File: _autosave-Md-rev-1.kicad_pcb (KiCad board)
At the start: 2 copper layers, 50 x 21.5 mm, 29 parts, among them J1 USB_C_Receptacle_USB2.0, J2 54-00177, U1 MCP73831-2-OT, U2 MAX9814

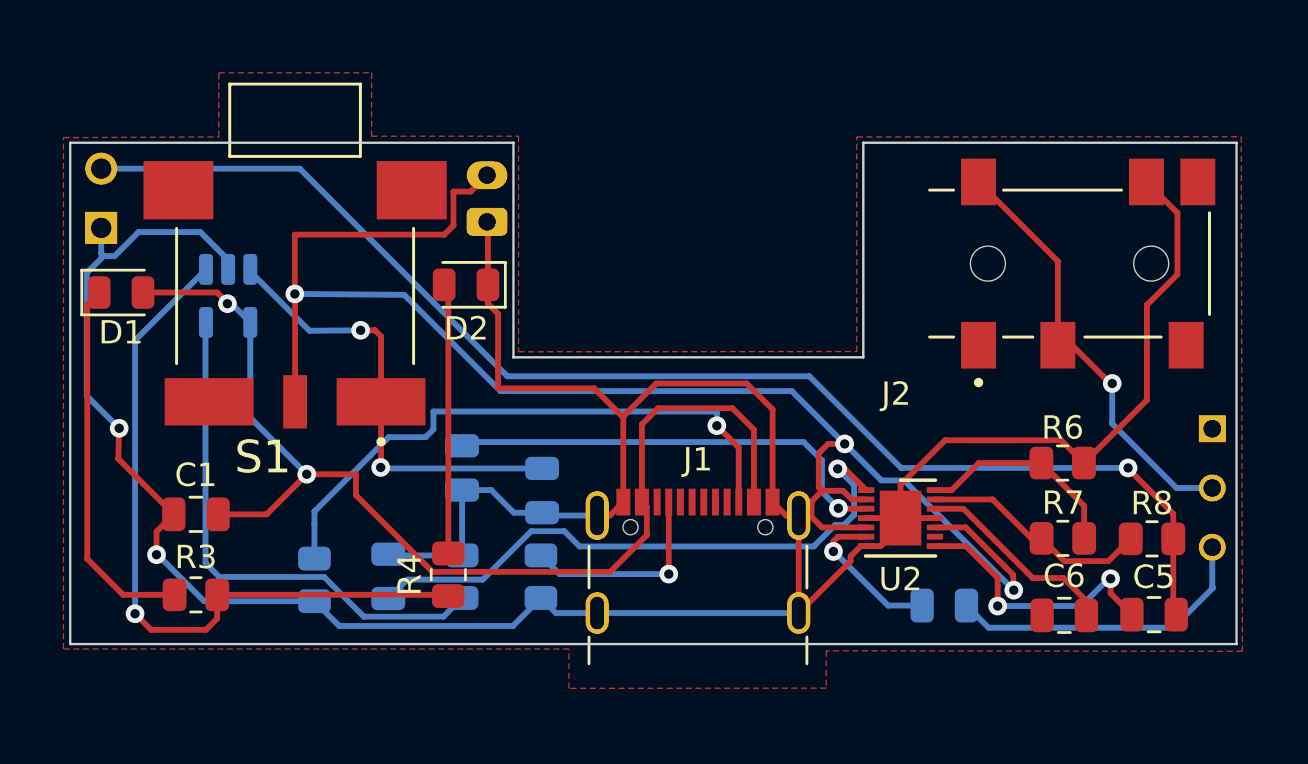
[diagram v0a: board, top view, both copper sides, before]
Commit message: updated the final PCB
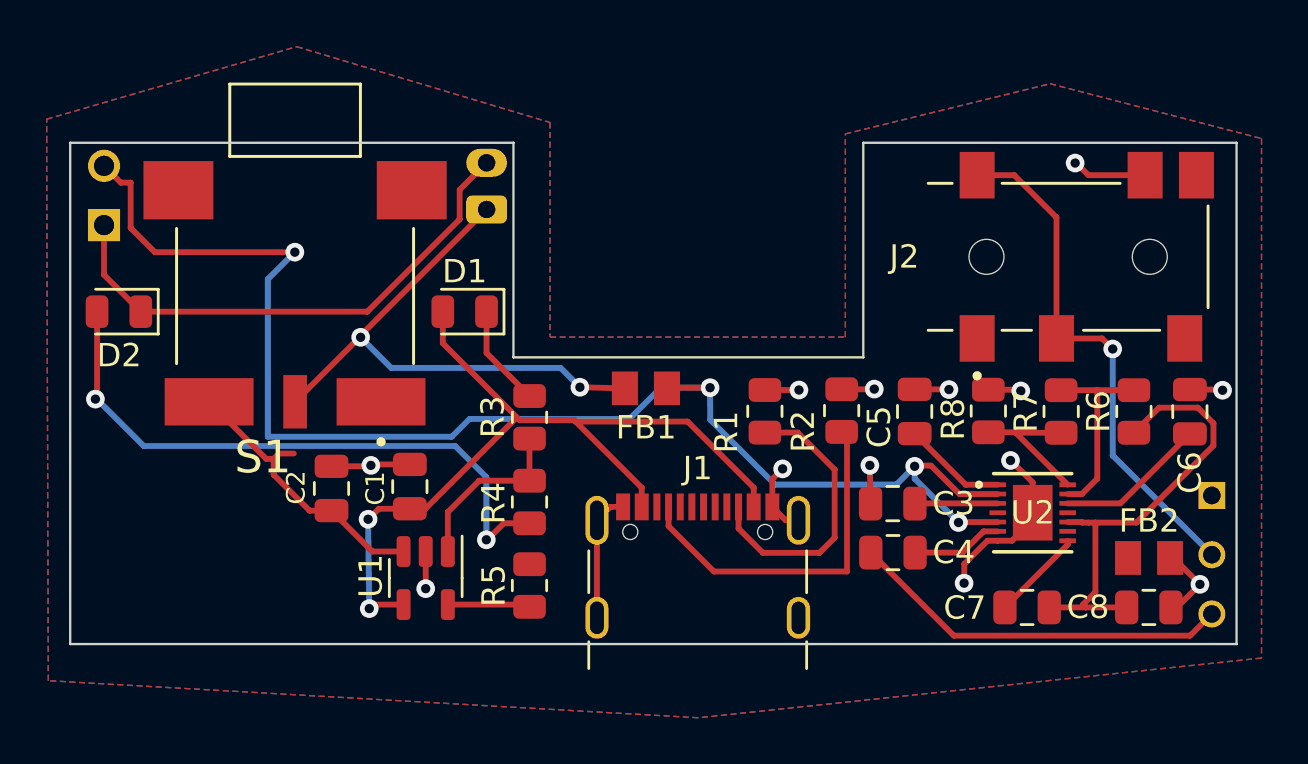
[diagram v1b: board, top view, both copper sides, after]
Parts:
- removed the ? at (179.0, 118.9)
- removed the ? at (147.9, 107.5)
- removed the ? at (179.0, 116.4)
- removed the ? at (131.3, 105.2)
- removed the ? at (179.0, 121.5)
- removed the ? at (147.9, 105.5)
- removed the ? at (131.3, 107.8)
- added ?: , , F.Cu at (178.9, 119.3)
- added ?: , , F.Cu at (178.9, 124.3)
- added ?: , , F.Cu at (131.4, 107.7)
- added ?: , , F.Cu at (147.8, 105.0)
- added ?: , , F.Cu at (131.4, 105.1)
- added ?: , , F.Cu at (147.8, 107.0)
- added ?: , , F.Cu at (178.9, 121.8)
- added C8: 2.2uF, Capacitor_SMD:C_0805_2012Metric, F.Cu at (176.2, 124.1)
- added FB1: FERRITE, LI0805H151R_10:IND_LI0805H151R-10_LRD, F.Cu at (154.7, 114.7)
- added FB2: FERRITE, LI0805H151R_10:IND_LI0805H151R-10_LRD, F.Cu at (176.2, 121.9)
- C2, R1, R2, R5, U1: moved to F.Cu
- C3: value 0.1uF -> 2.2uF; moved to F.Cu
- C4: value 2.2uF -> 10uF; moved to F.Cu
- C7: value 10uF -> 0.1uF; moved to F.Cu
- R6: value 100k -> 2.2K
- R8: value 2.2K -> 100k
- U2: value MAX9814 -> max9814etd+t; footprint Package_DFN_QFN:DFN-14-1EP_3x3mm_P0.4mm_EP1.78x2.35mm -> MAX9814etd+T:21-0137I_T1433-2_MXM
- moved C3 21.8 mm to (165.3, 119.6), turned to 0 degrees
- moved R1 20.6 mm to (159.8, 115.7), turned to 90 degrees
- moved C4 18.8 mm to (165.3, 121.7), turned to 0 degrees
- moved R3 16.2 mm to (149.7, 115.9), turned to 90 degrees
- moved D2 14.9 mm to (132.1, 111.4)
- moved U1 14.8 mm to (145.2, 122.8)
- moved D1 14.8 mm to (146.9, 111.4), turned to 180 degrees
- moved R2 14.7 mm to (163.1, 115.6), turned to 90 degrees
- moved C5 13.5 mm to (166.2, 115.7), turned to -90 degrees
- moved C6 10.3 mm to (178.0, 115.7), turned to -90 degrees
- moved C1 9.25 mm to (144.6, 118.9), turned to -90 degrees
- moved C2 9.03 mm to (141.2, 119.0), turned to 90 degrees
- moved R8 8.90 mm to (169.4, 115.6), turned to 90 degrees
- moved U2 5.67 mm to (171.3, 120.0)
- moved R7 5.44 mm to (172.5, 115.7), turned to -90 degrees
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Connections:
- C3 pad 2: Net-(U2-CT) -> Net-(U2-CG)
- C4 pad 1: GND -> /OUTPUT
- C4 pad 2: Net-(U2-CG) -> Net-(U2-MICOUT)
- C5 pad 1: Net-(C5-Pad1) -> GND
- C5 pad 2: Net-(U2-MICIN) -> Net-(U2-CT)
- C7 pad 1: Net-(U2-MICOUT) -> Net-(U2-MICIN)
- C7 pad 2: /OUTPUT -> VDD
- R6 pad 1: GND -> VDD
- R6 pad 2: Net-(U2-TH) -> Net-(U2-MICBIAS)
- R7 pad 1: Net-(U2-TH) -> Net-(U2-MICBIAS)
- R7 pad 2: Net-(U2-MICBIAS) -> Net-(U2-TH)
- R8 pad 1: Net-(C5-Pad1) -> Net-(U2-TH)
- R8 pad 2: Net-(U2-MICBIAS) -> GND
- S1 pad 1: Net-(U1-V_{BAT}) -> unconnected-(S1-Pad1)
- S1 pad 2: /GAIN -> /VBAT
- S1 pad 3: unconnected-(S1-Pad3) -> Net-(U1-V_{BAT})
- U2 pad 10: /GAIN -> VDD
- U2 pad 11: GND -> unconnected-(U2-NC-Pad11)
- U2 pad 2: /GAIN -> VDD
- U2 pad 4: GND -> unconnected-(U2-NC-Pad4)
- U2 pad 5: /GAIN -> VDD
- U2 pad 9: /A/R -> unconnected-(U2-A/R-Pad9)
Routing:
- net VDD: track 0.00 -> 81.8 mm, vias 0 -> 4
- net GND: track 134.2 -> 60.7 mm, vias 2 -> 13
- net /GAIN: track 67.5 -> 0.00 mm, vias 3 -> 0
- net Net-(C5-Pad1): track 57.0 -> 0.00 mm, vias 1 -> 0
- net /VBAT: track 0.00 -> 24.1 mm, vias 0 -> 2
- net Net-(U1-STAT): track 31.0 -> 7.55 mm, vias 1 -> 0
- net Net-(U2-CT): track 25.9 -> 4.47 mm, vias 1 -> 0
- net Net-(U1-PROG): track 22.6 -> 3.54 mm
- net Net-(U2-CG): track 19.4 -> 3.56 mm, vias 1 -> 0
- net Net-(D2-A): track 11.6 -> 27.0 mm, vias 0 -> 2
- net Net-(J1-CC2): track 25.8 -> 12.3 mm, vias 1 -> 0
- net /5V: track 48.6 -> 36.7 mm
- net Net-(D1-K): track 16.0 -> 4.38 mm
- net Net-(U2-MICIN): track 11.9 -> 3.97 mm, vias 2 -> 0
- net Net-(U1-V_{BAT}): track 19.5 -> 12.4 mm, vias 2 -> 0
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- added copper zone on B.Cu, net GND
